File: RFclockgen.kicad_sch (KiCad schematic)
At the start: 13 parts, among them J1 Conn_01x04_Pin, J3 Conn_01x02_Pin, U3 AP2112K-3.3, U4 ESP32-C6-WROOM-1-N8

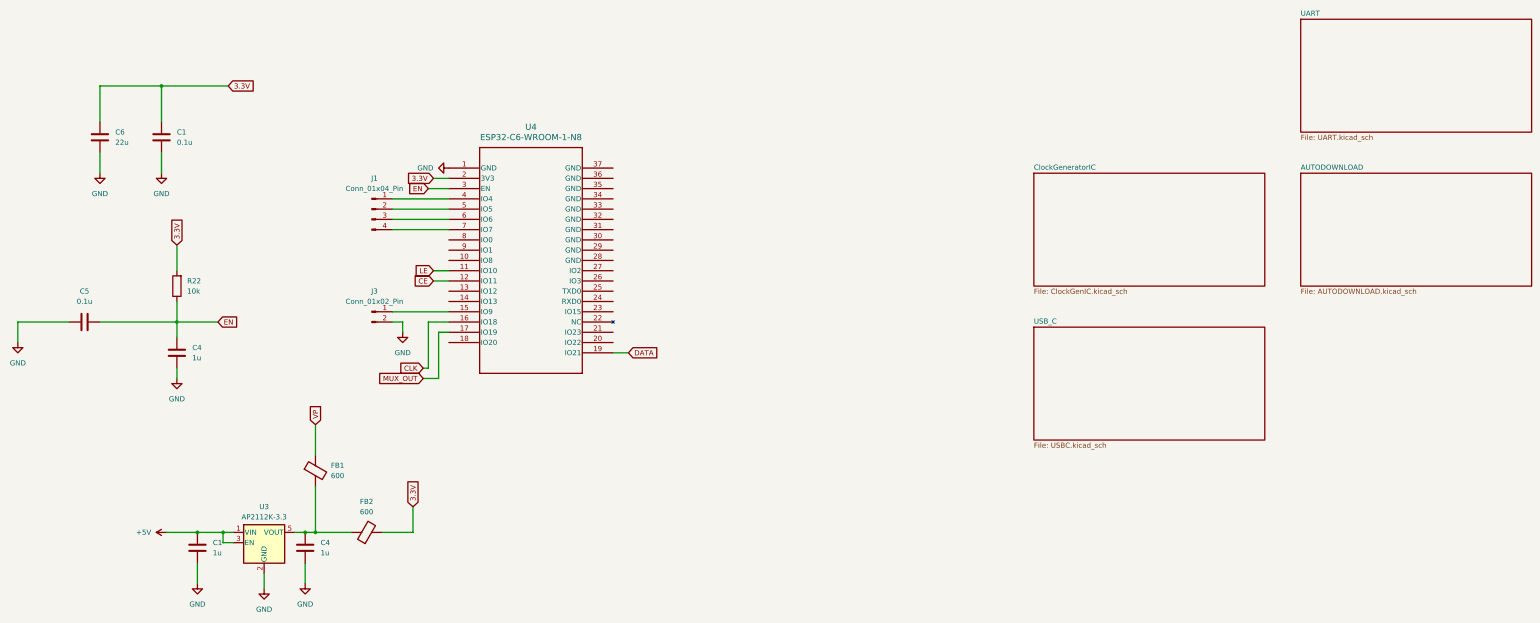
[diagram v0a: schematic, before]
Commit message: Update
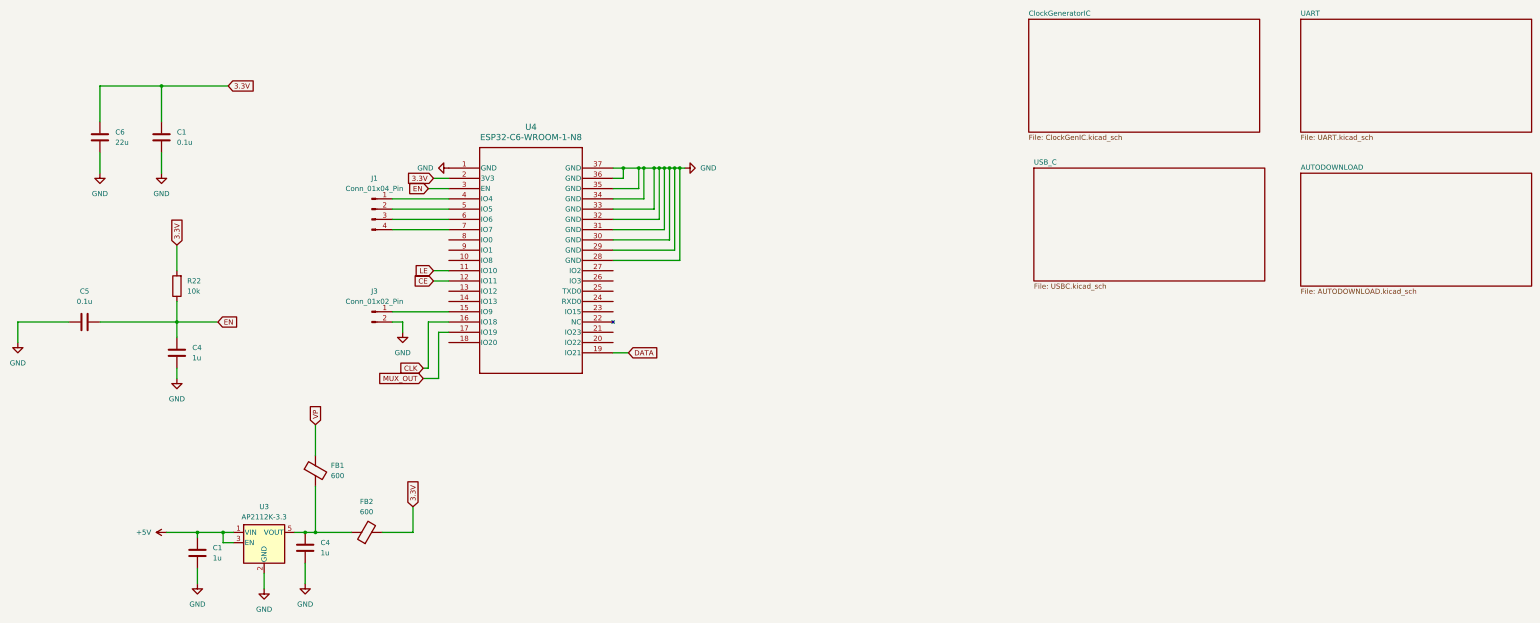
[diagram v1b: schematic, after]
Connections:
- net GND: now also U4.28 (GND), U4.29 (GND), U4.30 (GND), U4.31 (GND), U4.32 (GND), U4.33 (GND), U4.34 (GND), U4.35 (GND), U4.36 (GND), U4.37 (GND)
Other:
- moved on the sheet: C1
